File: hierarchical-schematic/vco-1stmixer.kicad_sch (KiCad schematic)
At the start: 44 parts, among them J101 VCO Control In, J102 1st IF Out, J103 VCO Sample, J104 RF In, J105 Conn_01x02, U101 POS-200, U102 MAV-11, U103 MAV-11, U104 TUF-1H+

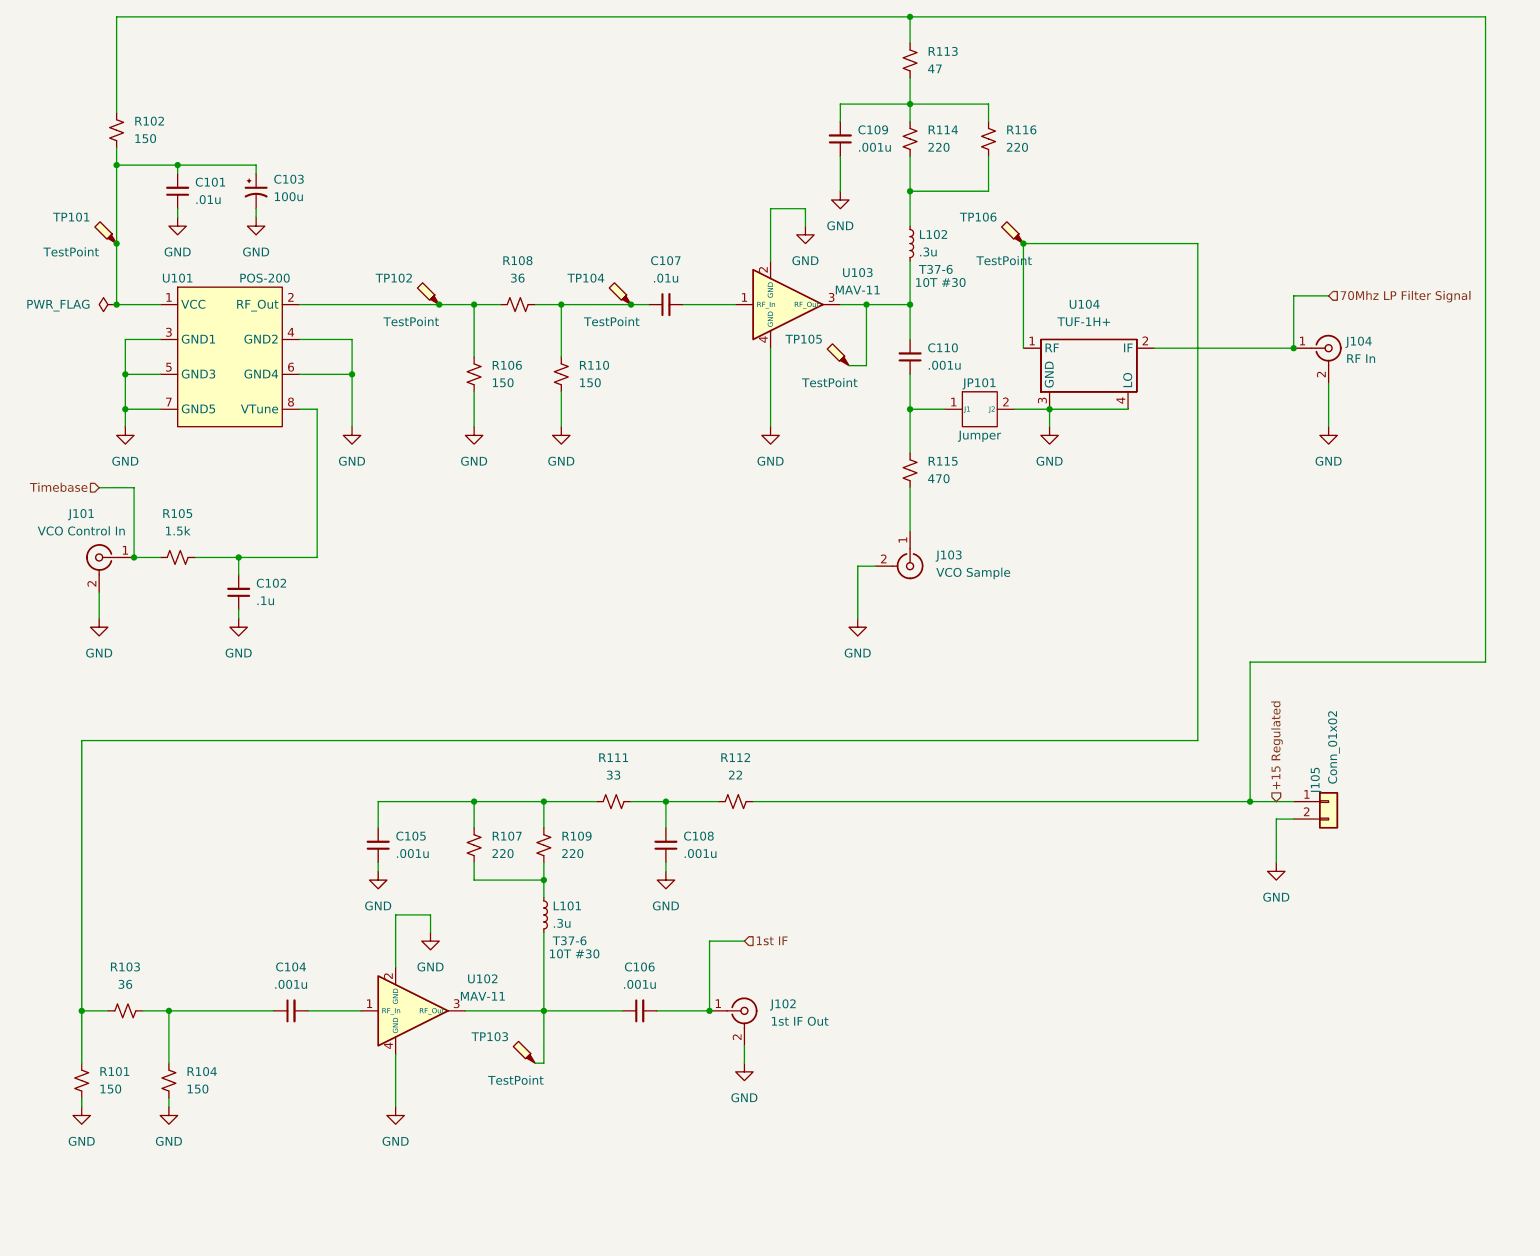
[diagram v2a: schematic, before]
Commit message: v7 conversion
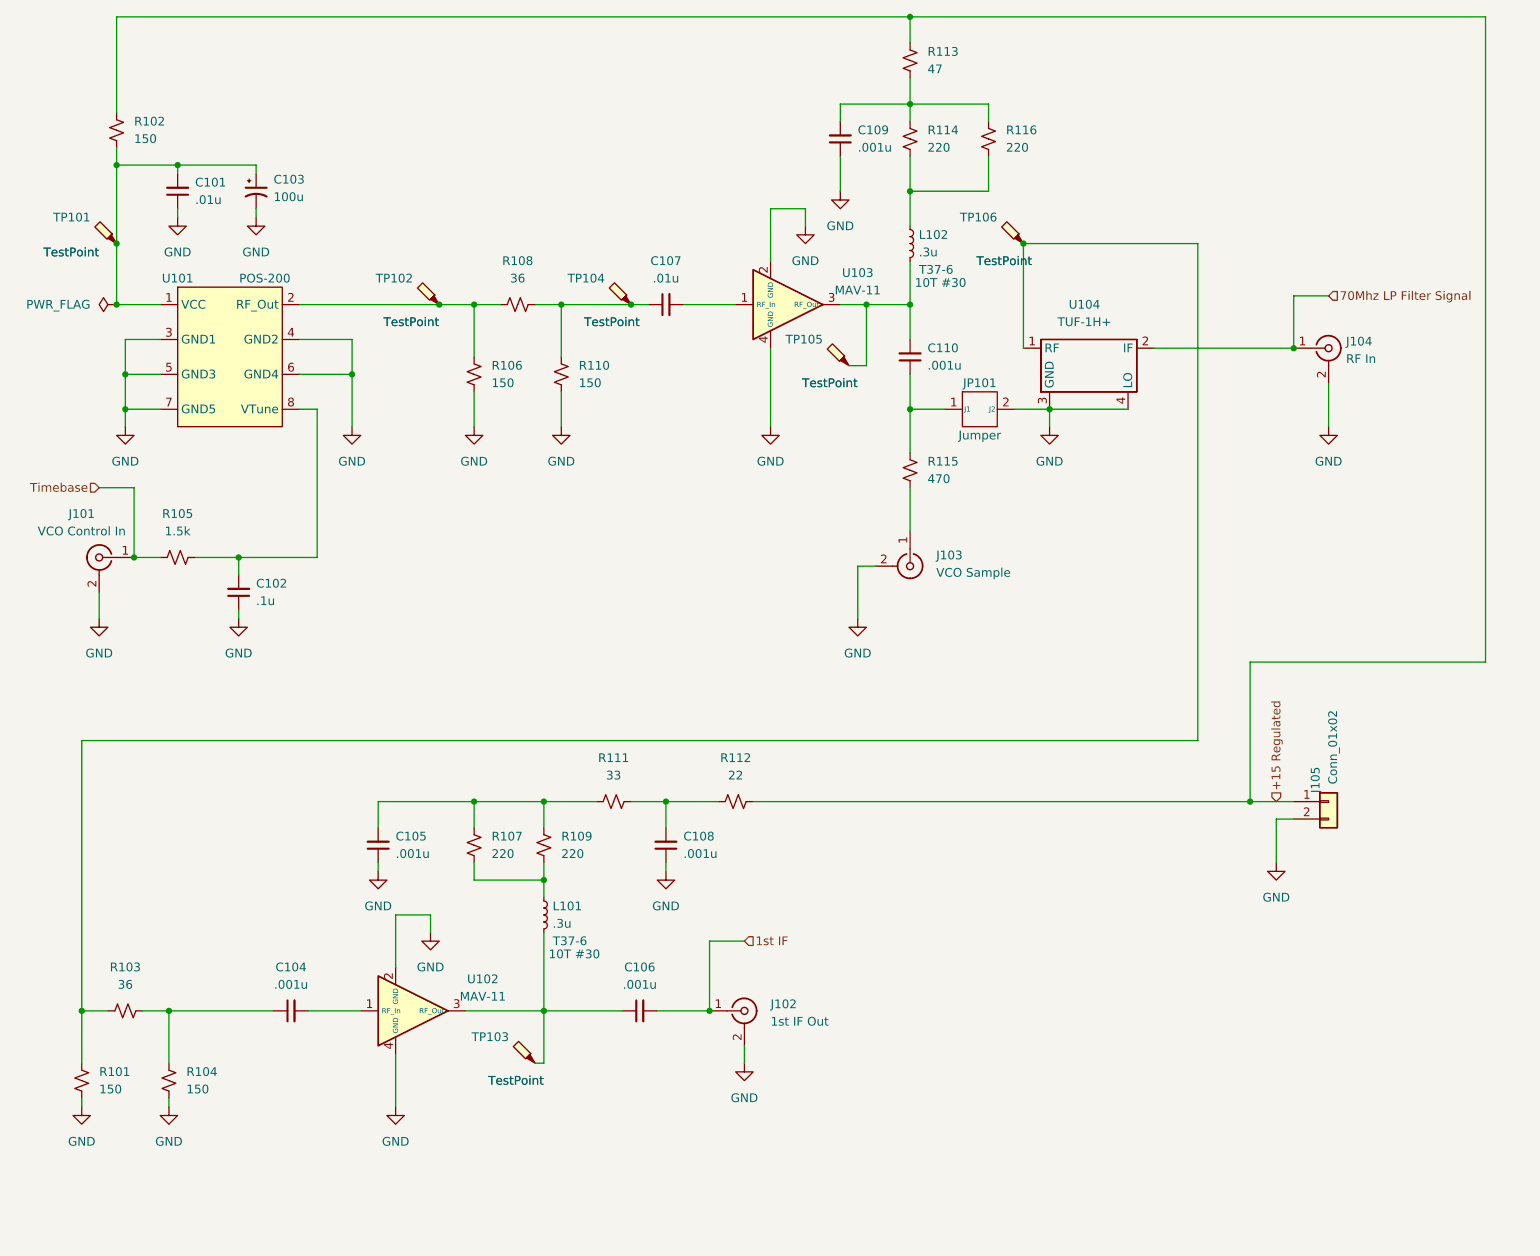
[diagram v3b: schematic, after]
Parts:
- J105: Spice_Model Conn_01x02 -> (none); Spice_Netlist_Enabled N -> (none); Spice_Primitive J -> (none)
- JP101: Spice_Model 22284028 -> (none); Spice_Netlist_Enabled N -> (none); Spice_Primitive J -> (none)
- TP101, TP102, TP103, TP104, TP105, TP106: value TestPoint -> ${SIM.PARAMS}; Spice_Netlist_Enabled N -> (none)
